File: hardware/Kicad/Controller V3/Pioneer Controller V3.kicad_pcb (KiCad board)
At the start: 2 copper layers, 72 x 98.8 mm, 27 parts, among them J1 Sensor Connector, J2 Power (IN), J4 Conn_Coaxial, SW1 SW_Push, SW2 SW_Push, SW5 SW_DIP_x02, U1 ESP32-S3, U2 2821, U3 DS3231_Precision_RTC, U4 RFM95W_LoRa_Radio_Transceiver, U5 BME280_Temperature_Sensor, U7 AP63205WU, U8 MicroSD_Breakout

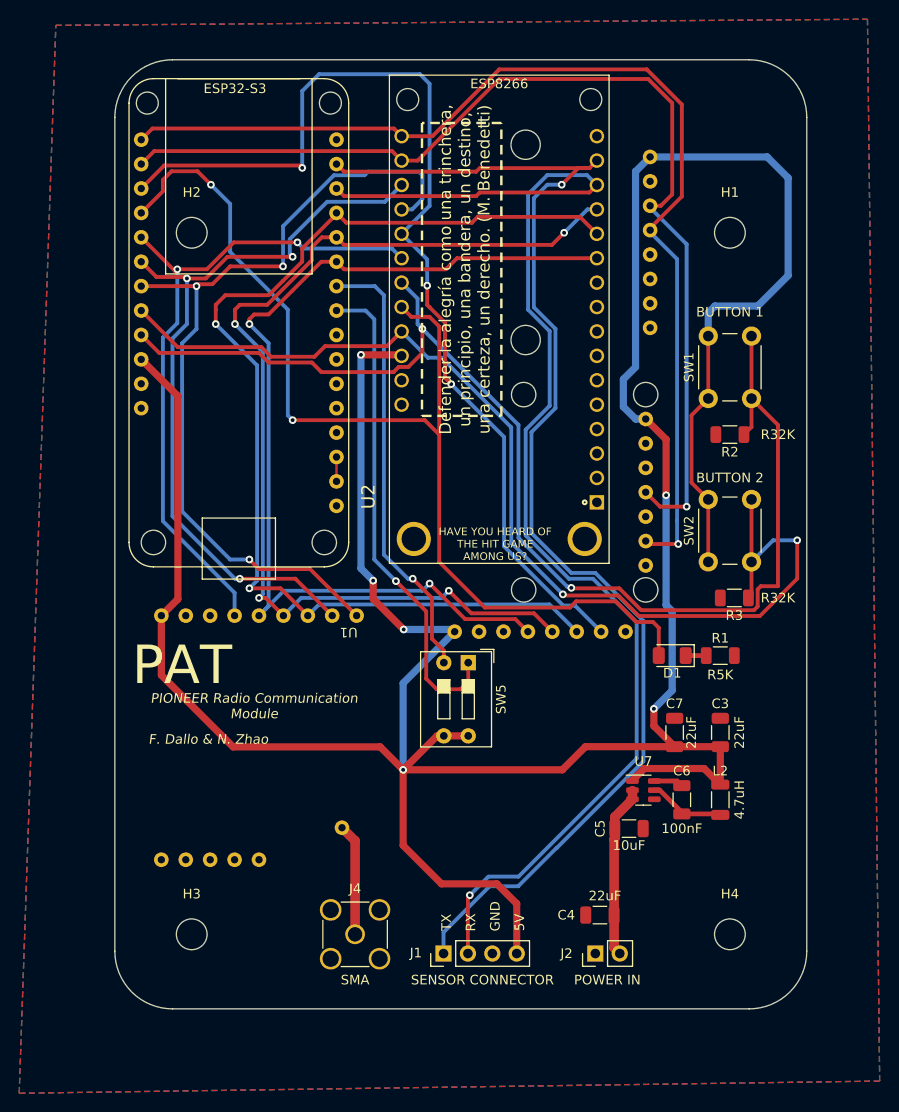
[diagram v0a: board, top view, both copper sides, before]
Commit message: more PCB updates
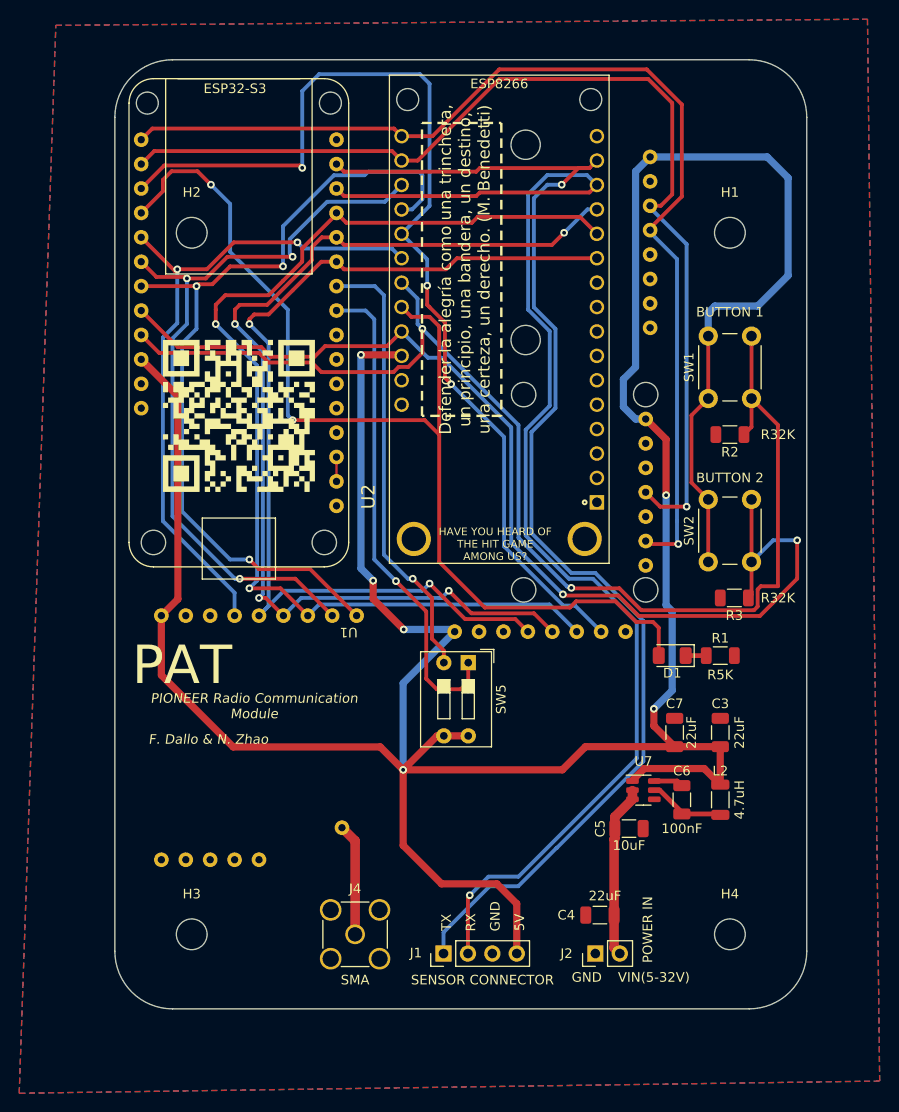
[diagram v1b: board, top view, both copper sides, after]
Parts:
- added G***: LOGO, LOGO, F.Cu at (41.9, 59.1)
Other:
- board text added: "VIN(5-32V)"
